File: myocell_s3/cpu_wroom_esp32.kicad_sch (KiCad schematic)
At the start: 21 parts, among them SW1 SW_Push, SW2 SW_Push, U4 ESP32-S3-WROOM-2

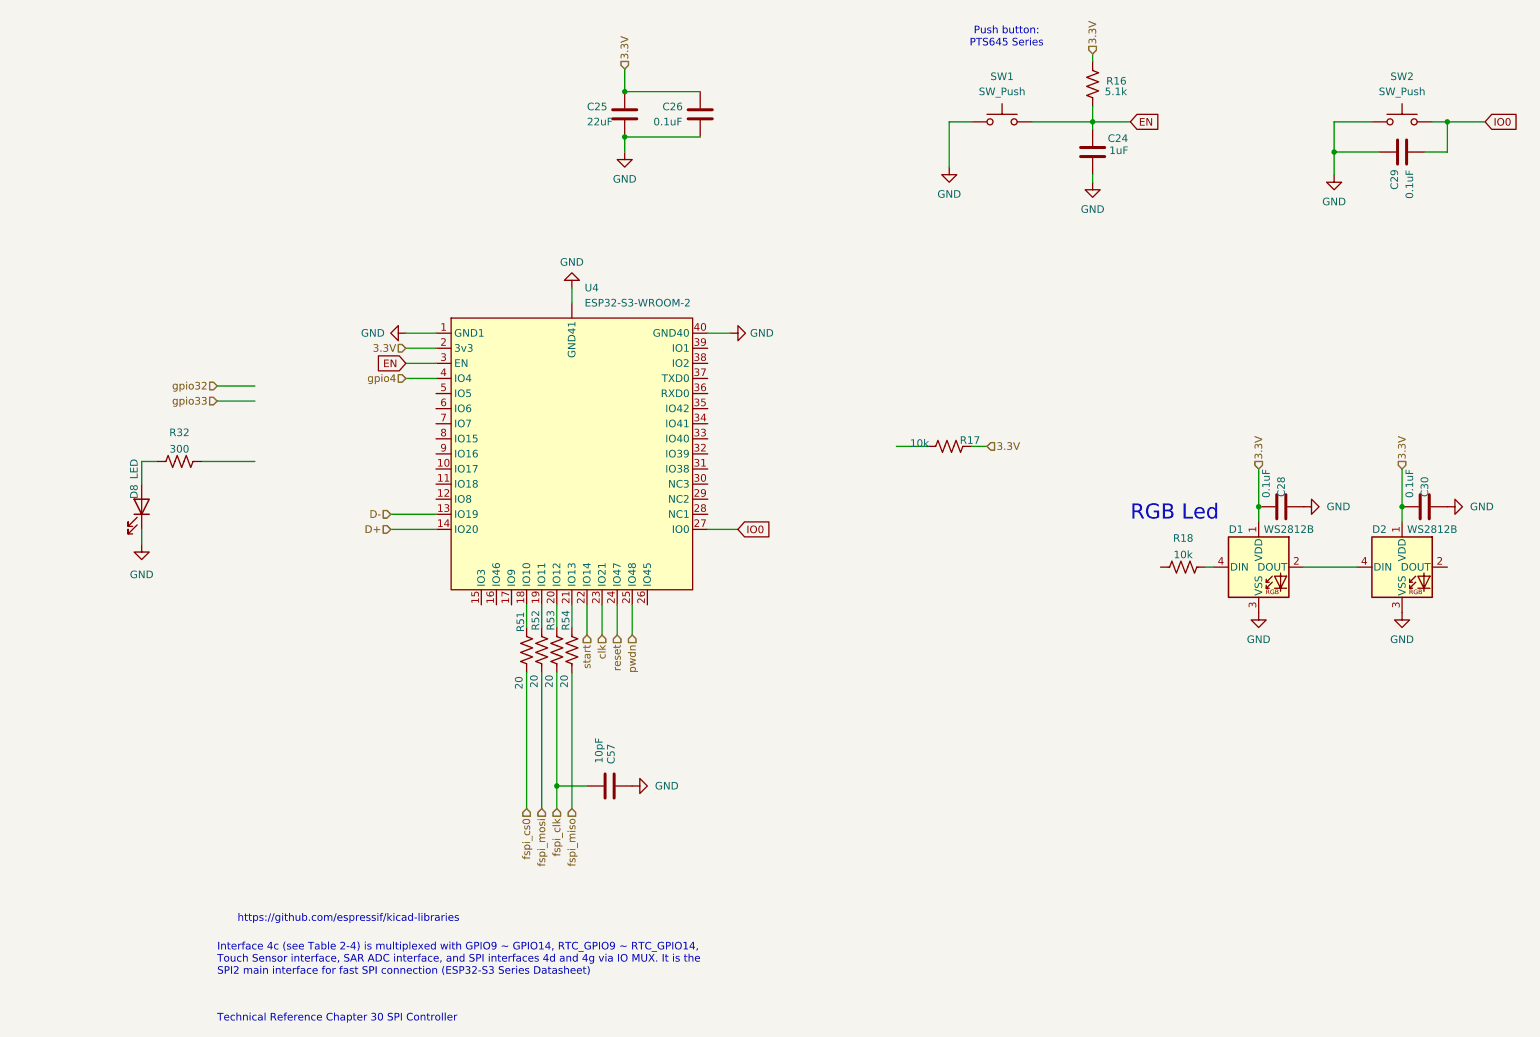
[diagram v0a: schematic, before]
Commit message: working on schematic transfer
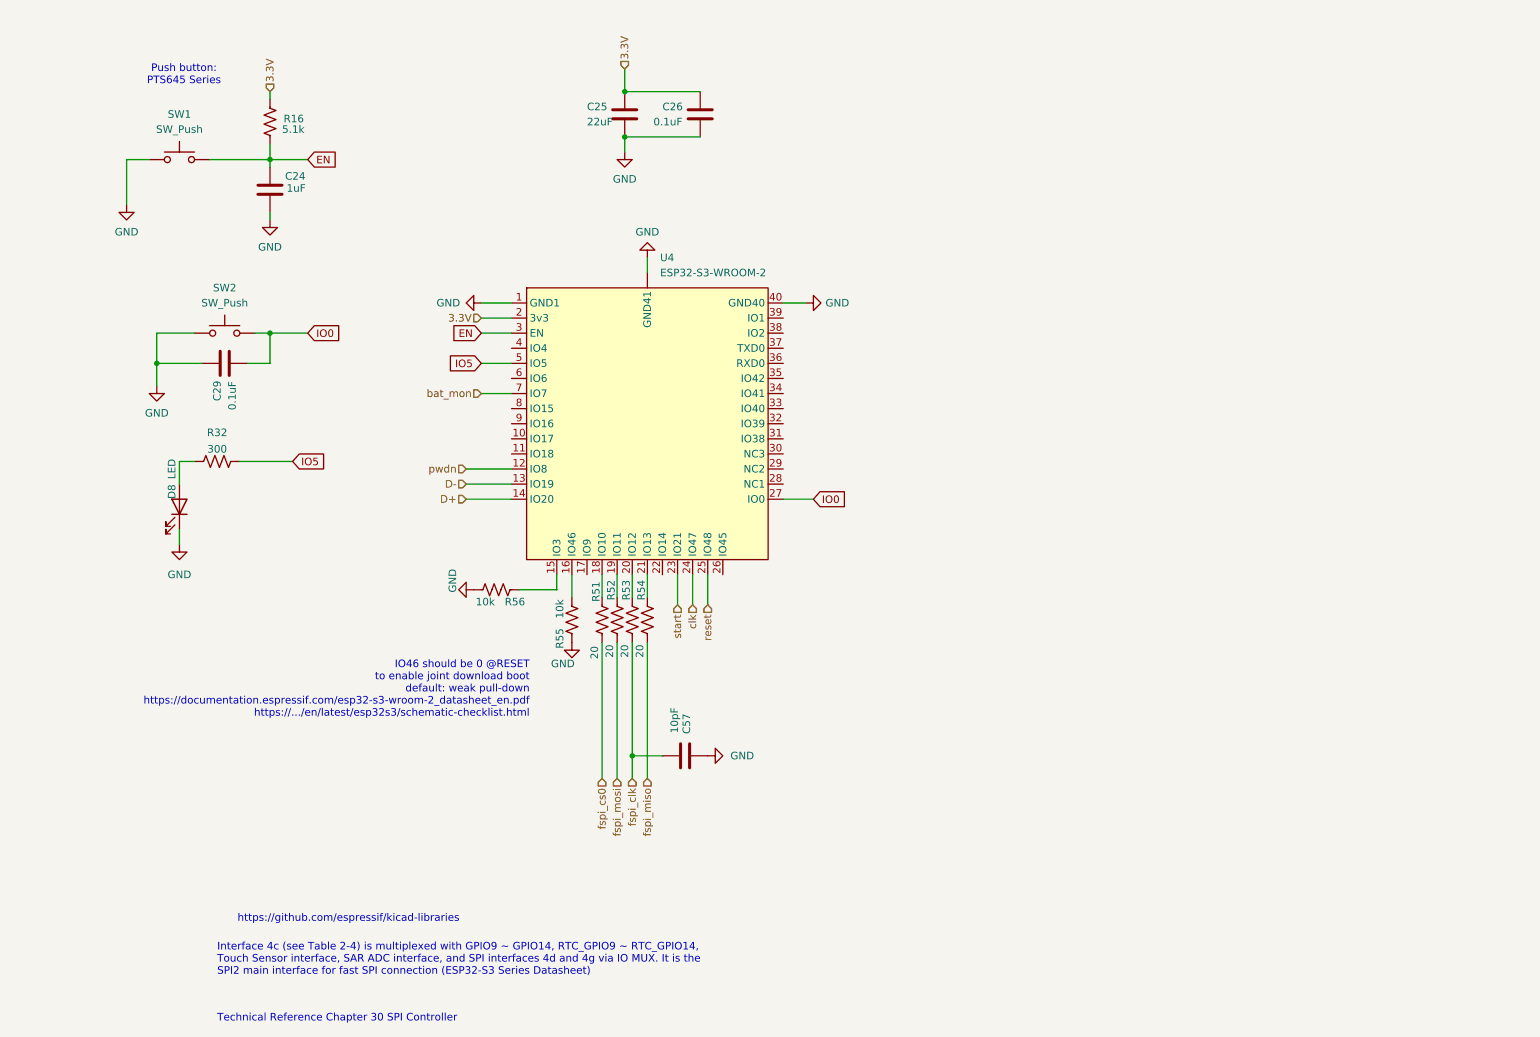
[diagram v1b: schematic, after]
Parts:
- removed C28, C30: 0.1uF, Capacitor_SMD:C_0805_2012Metric_Pad1.18x1.45mm_HandSolder, symbol Device:C
- removed D1, D2: WS2812B, LED_SMD:LED_WS2812B_PLCC4_5.0x5.0mm_P3.2mm, symbol LED:WS2812B
- removed R17, R18: 10k, Resistor_SMD:R_0805_2012Metric_Pad1.20x1.40mm_HandSolder, symbol Device:R_US
- added R55, R56: 10k, Resistor_SMD:R_0805_2012Metric_Pad1.20x1.40mm_HandSolder, symbol Device:R_US
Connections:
- net GND: now also R55.1, R56.2
- net clk: now also U4.24 (IO47); no longer U4.23 (IO21)
- net pwdn: now also U4.12 (IO8); no longer U4.25 (IO48)
- net reset: now also U4.25 (IO48); no longer U4.24 (IO47)
- net start: now also U4.23 (IO21); no longer U4.22 (IO14)
- net IO5: now reaches R32.2
- net IO5: now also U4.5 (IO5)
- net at U4.15 (IO3): now also R56.1
- net at U4.16 (IO46): now also R55.2
- net bat_mon: now reaches U4.7 (IO7)
- net gpio4: no longer names the net of U4.4 (IO4)
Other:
- note added: "IO46 should be 0 @RESET to enable joint download boot default: weak pull-down https://documentation.espressif.com/esp32-s3-wroom-2_datasheet_en.pdf https://.../en/latest/esp32s3/schematic-checklist.html"
- note removed: "RGB Led"
- moved on the sheet: C24, C29, C57, D8, R16, R32, R51, R52, R53, R54, SW1, SW2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
